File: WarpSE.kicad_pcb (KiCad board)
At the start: 4 copper layers, 109.1 x 102.1 mm, 123 parts, among them J1 MacSEPDS, J2 JTAG, J3 microUSB, Q1 MMBT3904, Q2 MMBT3904, Q3 MMBT3904, Q4 MMBT3904, U1 XC95144XL-TQ100, U10 39SF040, U11 39SF040, U12 CH340G, U13 74AHCT573PW, U14 MC68HC000FN20, U15 74AHCT573PW, U16 74AHCT573PW, U17 74AHCT573PW, U18 74AHCT573PW, U19 74AHCT573PW, U2 74AHCT573PW, U20 74AHCT573PW, U21 74AHCT573PW, U22 74AHCT573PW, U23 74AHCT573PW, U24 74AHCT573PW, U25 74LVC245APW, U26 74LVC1G07GW, U27 74LVC1G07GW, U28 74LVC1G07GW, U3 AZ1117EH-3.3, U4 DNP-AZ1117CH2-3.3, U5 50M, U6 74LVC1G74DC, U7 74LVC1G74DC, U8 KM48C2100, U9 KM48C2100, Y1 12M

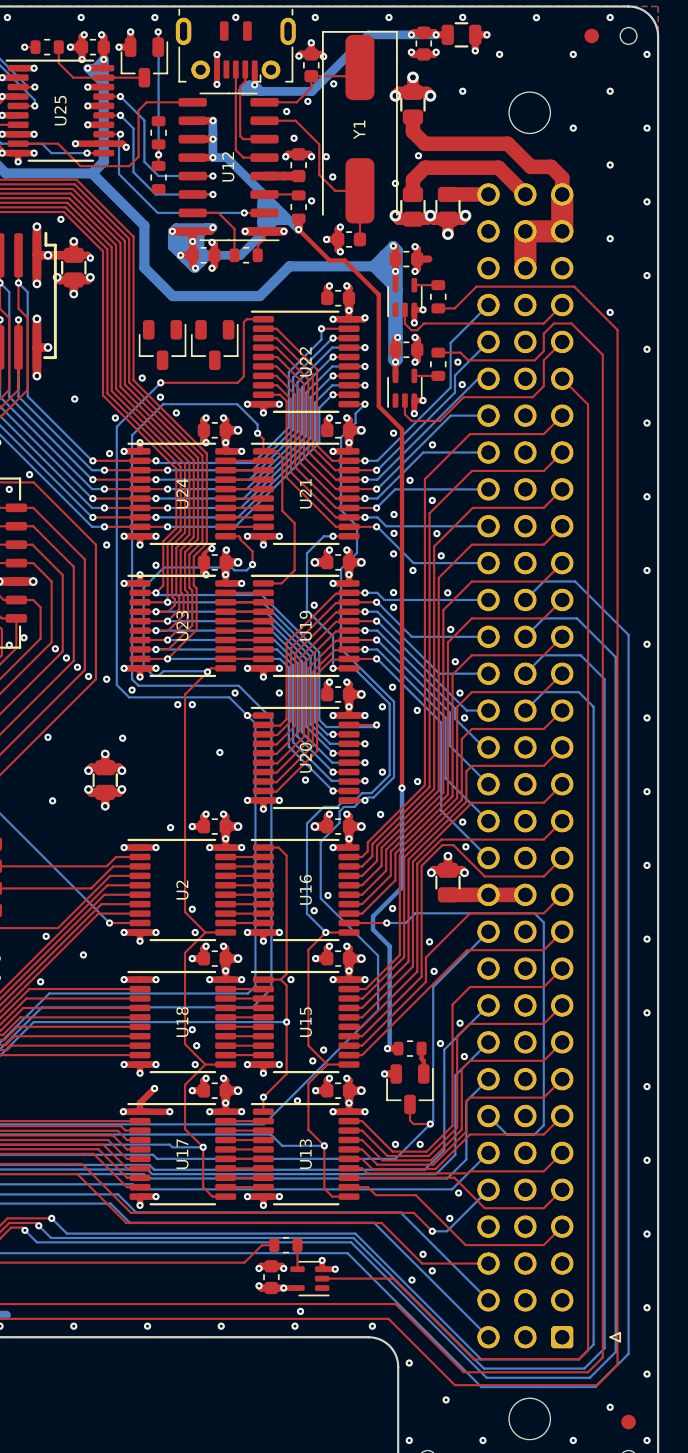
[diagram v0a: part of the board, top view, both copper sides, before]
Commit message: Revert "idk"
This reverts commit aa30aa8a559ae1d3e965923a55380a6d00f93ea4.
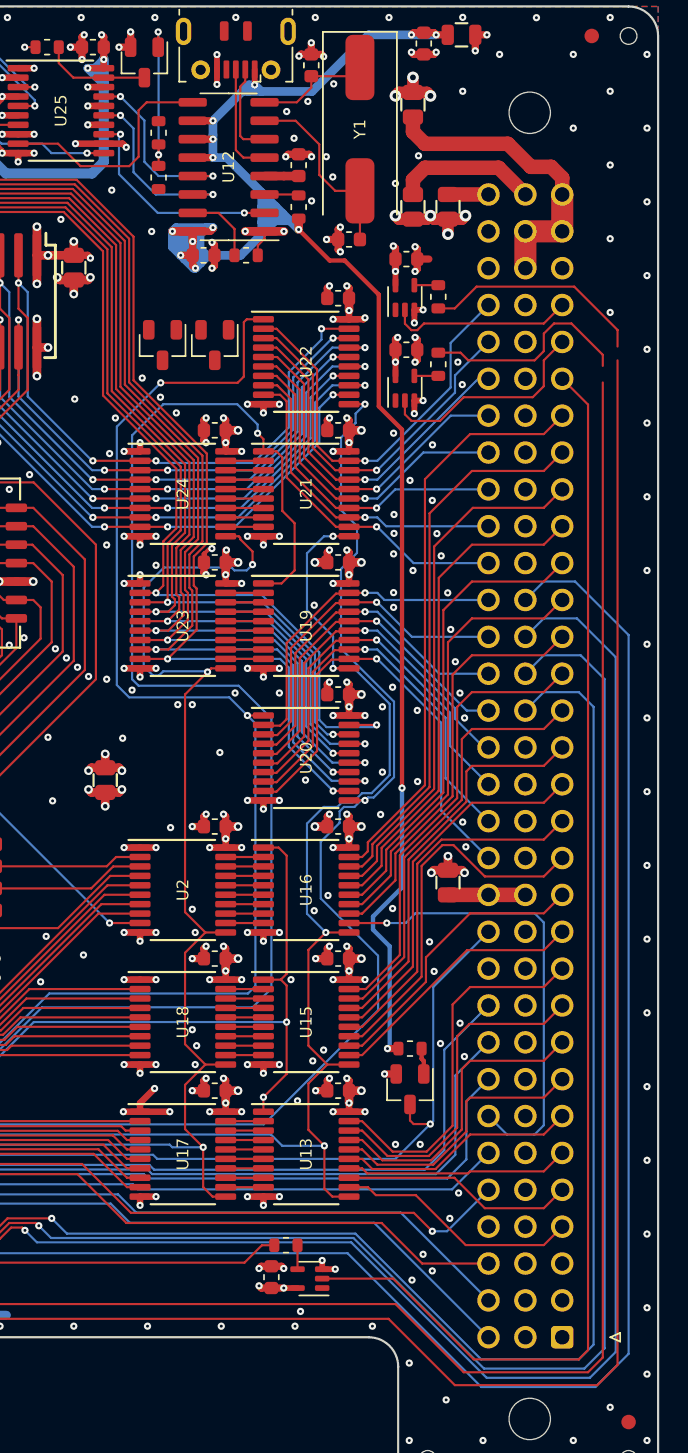
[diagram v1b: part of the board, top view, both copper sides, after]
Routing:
- net +3V3: track 450.3 -> 402.6 mm
- net USB5V: track 139.7 -> 142.5 mm
- net /ClkBuf/BC8M: track 181.0 -> 179.8 mm
- net /ClkBuf/BC16M: track 184.5 -> 183.6 mm
- net GND: vias 699 -> 701
